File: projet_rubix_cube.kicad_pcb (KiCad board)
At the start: 2 copper layers, 24 parts, among them J1 Screw_Terminal_01x04, J2 Screw_Terminal_01x04, J3 Screw_Terminal_01x03, U2 L298HN

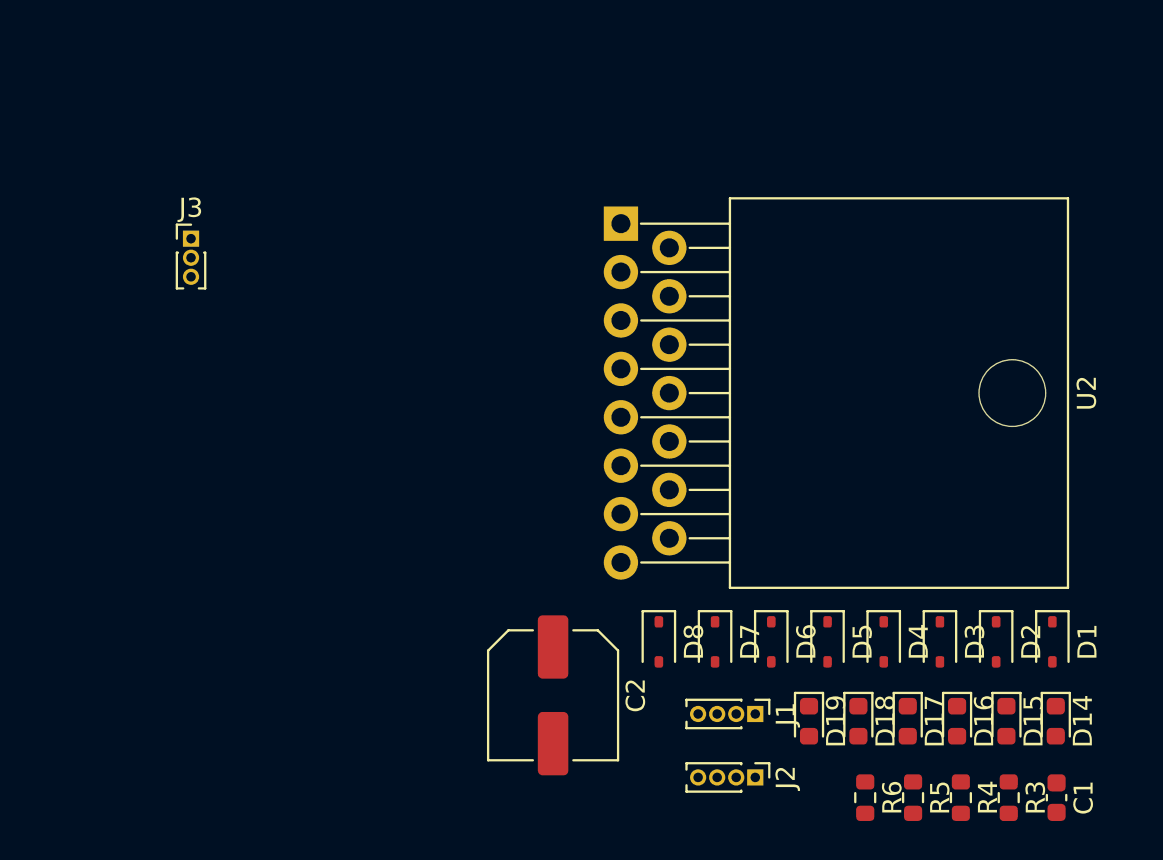
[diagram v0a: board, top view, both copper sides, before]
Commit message: routage_carte
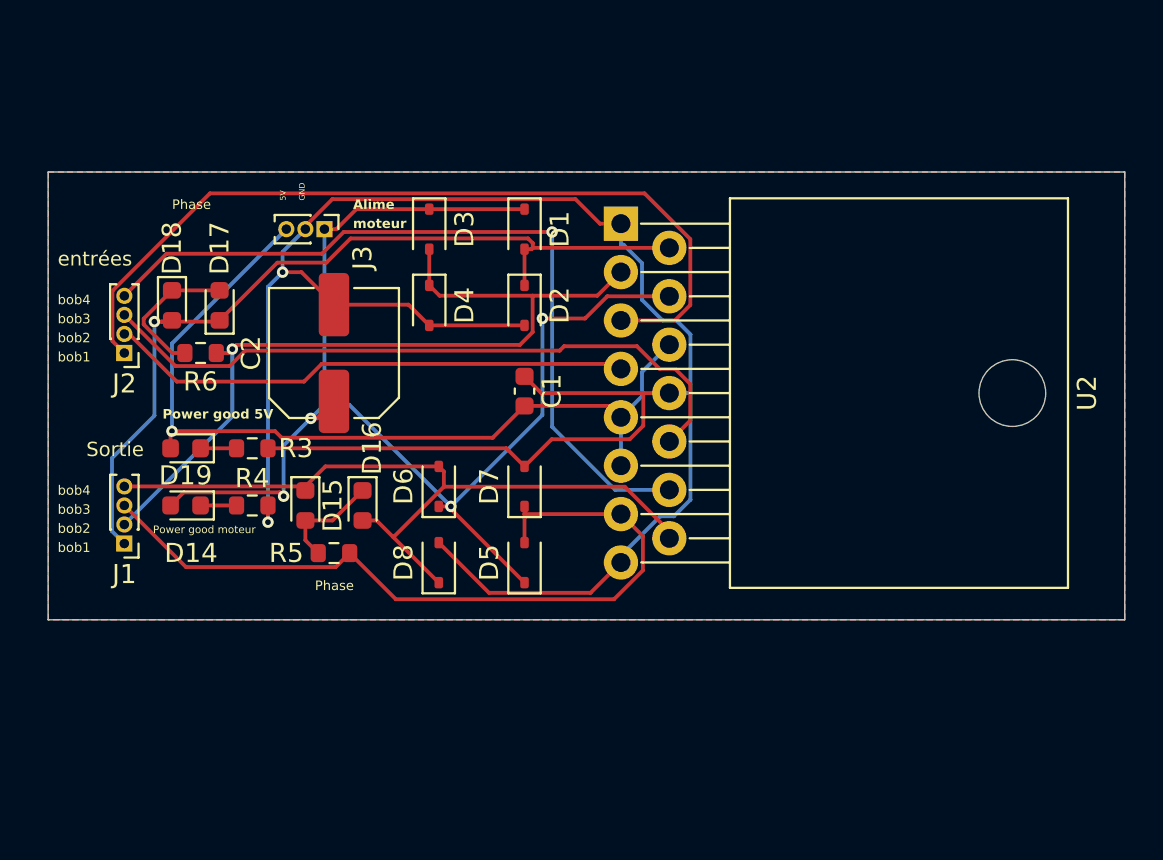
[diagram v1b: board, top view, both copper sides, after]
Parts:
- moved D14 47.1 mm to (128.2, 54.5), turned to 180 degrees
- moved R3 43.7 mm to (131.7, 51.5), turned to 0 degrees
- moved D17 42.2 mm to (130.0, 44.0), turned to 90 degrees
- moved D18 42.1 mm to (127.5, 44.0)
- moved R6 42.0 mm to (129.0, 46.5), turned to 0 degrees
- moved R4 40.2 mm to (131.7, 54.5), turned to 0 degrees
- moved J2 39.9 mm to (125.0, 46.5), turned to 180 degrees
- moved D15 38.5 mm to (134.5, 54.5)
- moved D19 35.7 mm to (128.2, 51.5), turned to 180 degrees
- moved D1 35.2 mm to (146.0, 40.0)
- moved C1 35.1 mm to (146.0, 48.5)
- moved D3 34.5 mm to (141.0, 40.0)
- moved J1 34.3 mm to (125.0, 56.5), turned to 180 degrees
- moved D16 33.2 mm to (137.5, 54.5)
- moved R5 33.0 mm to (136.0, 57.0), turned to 0 degrees
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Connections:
- J2 pad 1: alim_bobine2 -> alim_bobine1
- J2 pad 2: alim_bobine1 -> alim_bobine2
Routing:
- net GND: track 0.00 -> 113.6 mm, vias 0 -> 2
- net +24V: track 0.00 -> 67.8 mm, vias 0 -> 4
- net +5V: track 0.00 -> 46.1 mm, vias 0 -> 1
- net out_bobine1: track 0.00 -> 44.9 mm, vias 0 -> 1
- net alim_bobine1: track 0.00 -> 44.4 mm
- net out_bobine2: track 0.00 -> 43.2 mm, vias 0 -> 1
- net alim_bobine4: track 0.00 -> 41.6 mm, vias 0 -> 1
- net out_bobine3: track 0.00 -> 40.9 mm
- net out_bobine4: track 0.00 -> 40.6 mm
- net alim_bobine3: track 0.00 -> 35.5 mm
- net alim_bobine2: track 0.00 -> 27.6 mm
- net Net-(D17-A): track 0.00 -> 7.69 mm
- net Net-(D15-A): track 0.00 -> 5.64 mm
- net Net-(D19-K): track 0.00 -> 1.89 mm
- net Net-(D14-K): track 0.00 -> 1.89 mm
- added copper zone on B.Cu, net GND
- added copper zone on F.Cu, net GND
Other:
- board outline added: 56.5 x 23.5 mm
- board text added: "5V"
- board text added: "Alime"
- board text added: "GND"
- board text added: "Phase"
- board text added: "Power good 5V"
- board text added: "Power good moteur"
- board text added: "Sortie"
- board text added: "bob1"
- board text added: "bob2"
- board text added: "bob3"
- board text added: "bob4"
- board text added: "entrées"
- board text added: "moteur"

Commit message: New rules
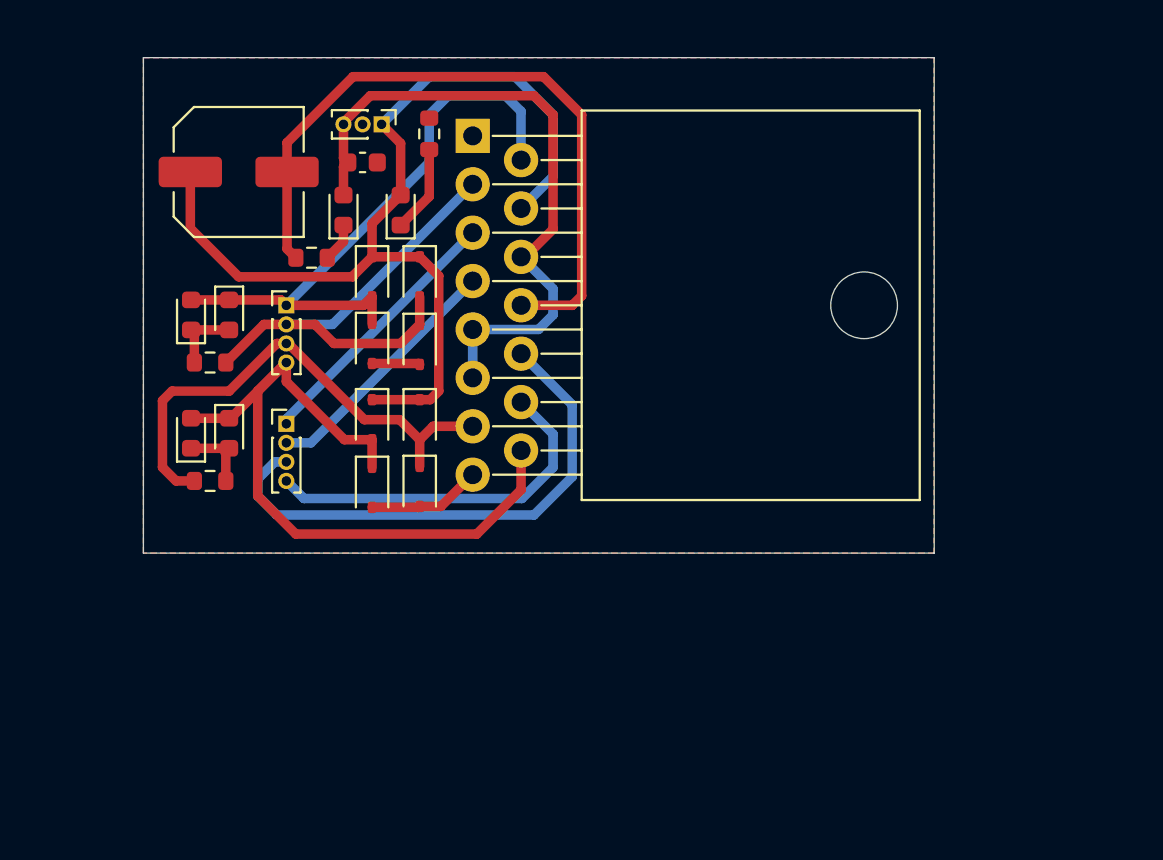
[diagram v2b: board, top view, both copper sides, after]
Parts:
- moved R4 21.6 mm to (141.0, 35.0), turned to 90 degrees
- moved D14 19.2 mm to (139.5, 39.0), turned to 90 degrees
- moved J1 15.1 mm to (133.5, 44.0), turned to 0 degrees
- moved D19 15.0 mm to (136.5, 39.0), turned to 90 degrees
- moved C1 14.7 mm to (137.5, 36.5), turned to 180 degrees
- moved C2 10.7 mm to (131.0, 37.0), turned to 0 degrees
- moved R3 10.5 mm to (134.8, 41.5), turned to 180 degrees
- moved D16 9.76 mm to (128.5, 50.7), turned to 90 degrees
- moved D5 9.30 mm to (140.5, 50.0), turned to -90 degrees
- moved J2 9.28 mm to (133.5, 50.2), turned to 0 degrees
- moved U2 9.04 mm to (143.3, 35.1)
- moved D1 8.38 mm to (138.0, 42.5)
- moved D2 8.25 mm to (138.0, 46.0)
- moved R5 7.52 mm to (129.5, 53.2), turned to 180 degrees
- moved J3 6.26 mm to (138.5, 34.5)
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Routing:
- net GND: track 113.6 -> 45.4 mm, vias 2 -> 0
- net alim_bobine1: track 44.4 -> 14.1 mm
- net alim_bobine4: track 41.6 -> 19.2 mm, vias 1 -> 0
- net out_bobine2: track 43.2 -> 26.1 mm, vias 1 -> 0
- net +24V: track 67.8 -> 52.1 mm, vias 4 -> 0
- net alim_bobine2: track 27.6 -> 13.3 mm
- net out_bobine3: track 40.9 -> 26.8 mm
- net out_bobine1: track 44.9 -> 32.4 mm, vias 1 -> 0
- net +5V: track 46.1 -> 35.1 mm, vias 1 -> 0
- net alim_bobine3: track 35.5 -> 28.1 mm
- net Net-(D17-A): track 7.69 -> 3.78 mm
- net Net-(D14-K): track 1.89 -> 4.58 mm
- net Net-(D15-A): track 5.64 -> 3.78 mm
- net out_bobine4: track 40.6 -> 39.7 mm
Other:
- board size 56.5 x 23.5 mm -> 41.5 x 26 mm
- board text added: "Q.G"
- board text removed: "5V"
- board text removed: "Alime"
- board text removed: "GND"
- board text removed: "Phase"
- board text removed: "Power good 5V"
- board text removed: "Power good moteur"
- board text removed: "Sortie"
- board text removed: "bob1"
- board text removed: "bob2"
- board text removed: "bob3"
- board text removed: "bob4"
- board text removed: "entrées"
- board text removed: "moteur"

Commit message: DRC OK
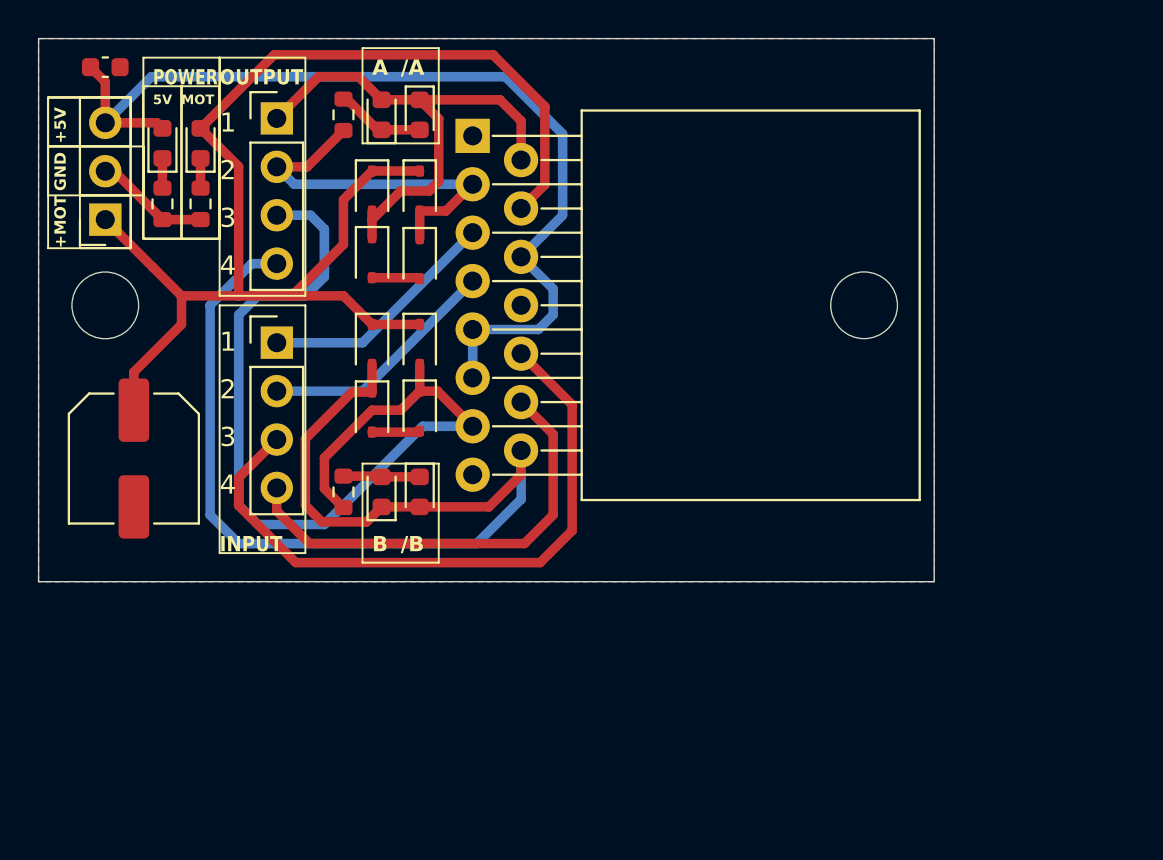
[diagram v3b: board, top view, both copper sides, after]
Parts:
- added ?: , , F.Cu at (124.0, 44.0)
- J1, J2: footprint Connector_PinHeader_1.00mm:PinHeader_1x04_P1.00mm_Vertical -> Connector_PinHeader_2.54mm:PinHeader_1x04_P2.54mm_Vertical
- J3: footprint Connector_PinHeader_1.00mm:PinHeader_1x03_P1.00mm_Vertical -> Connector_PinSocket_2.54mm:PinSocket_1x03_P2.54mm_Vertical
- moved C2 16.0 mm to (125.5, 52.0), turned to -90 degrees
- moved J3 15.3 mm to (124.0, 39.5), turned to 180 degrees
- moved R6 14.8 mm to (136.5, 34.0), turned to -90 degrees
- moved D17 14.5 mm to (140.5, 34.0)
- moved D18 14.5 mm to (138.5, 34.0)
- moved C1 14.4 mm to (124.0, 31.5)
- moved R4 12.6 mm to (129.0, 38.7), turned to -90 degrees
- moved D16 12.4 mm to (140.5, 53.8), turned to -90 degrees
- moved D14 11.1 mm to (129.0, 35.5)
- moved D19 10.1 mm to (127.0, 35.5)
- moved J1 9.82 mm to (133.0, 34.2)
- moved D15 8.57 mm to (138.5, 53.8), turned to 90 degrees
- moved R3 8.32 mm to (127.0, 38.7), turned to -90 degrees
- moved R5 7.02 mm to (136.5, 53.8), turned to -90 degrees
- moved D1 4.50 mm to (138.0, 38.0)
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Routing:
- net GND: track 45.4 -> 11.1 mm
- net out_bobine3: track 26.8 -> 49.9 mm
- net +24V: track 52.1 -> 72.9 mm
- net out_bobine4: track 39.7 -> 59.3 mm
- net +5V: track 35.1 -> 50.8 mm
- net out_bobine2: track 26.1 -> 19.8 mm
- net alim_bobine3: track 28.1 -> 34.1 mm
- net out_bobine1: track 32.4 -> 27.2 mm
- net alim_bobine4: track 19.2 -> 23.7 mm
- net Net-(D14-K): track 4.58 -> 1.56 mm
- net alim_bobine1: track 14.1 -> 12.7 mm
- net Net-(D17-A): track 3.78 -> 4.67 mm
- net alim_bobine2: track 13.3 -> 12.7 mm
- net Net-(D19-K): track 2.06 -> 1.56 mm
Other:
- board size 41.5 x 26 mm -> 47 x 28.5 mm
- board text added: "+5V"
- board text added: "+MOT"
- board text added: "/A"
- board text added: "/B"
- board text added: "1"
- board text added: "2"
- board text added: "3"
- board text added: "4"
- board text added: "5V MOT"
- board text added: "A"
- board text added: "B"
- board text added: "GND"
- board text added: "INPUT"
- board text added: "OUTPUT"
- board text added: "POWER"
